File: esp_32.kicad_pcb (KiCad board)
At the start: 4 copper layers, 96 x 54 mm, 90 parts, among them J1 SS-52400-002, J3 GSD090012SEU, J4 B4B-XH-AM, J5 B2B-PH-SM4-TB, J6 Conn_01x05, Q1 TEMT6000X01, Q2 BC817, Q3 BC817, U1 MCP73871, U2 BME280, U3 ESP32-C3-WROOM-02-H4, U4 CP2102N-Axx-xQFN20, U5 USBLC6-2SC6, U6 W25Q32JVSSIQ, U7 MAX4466EXK

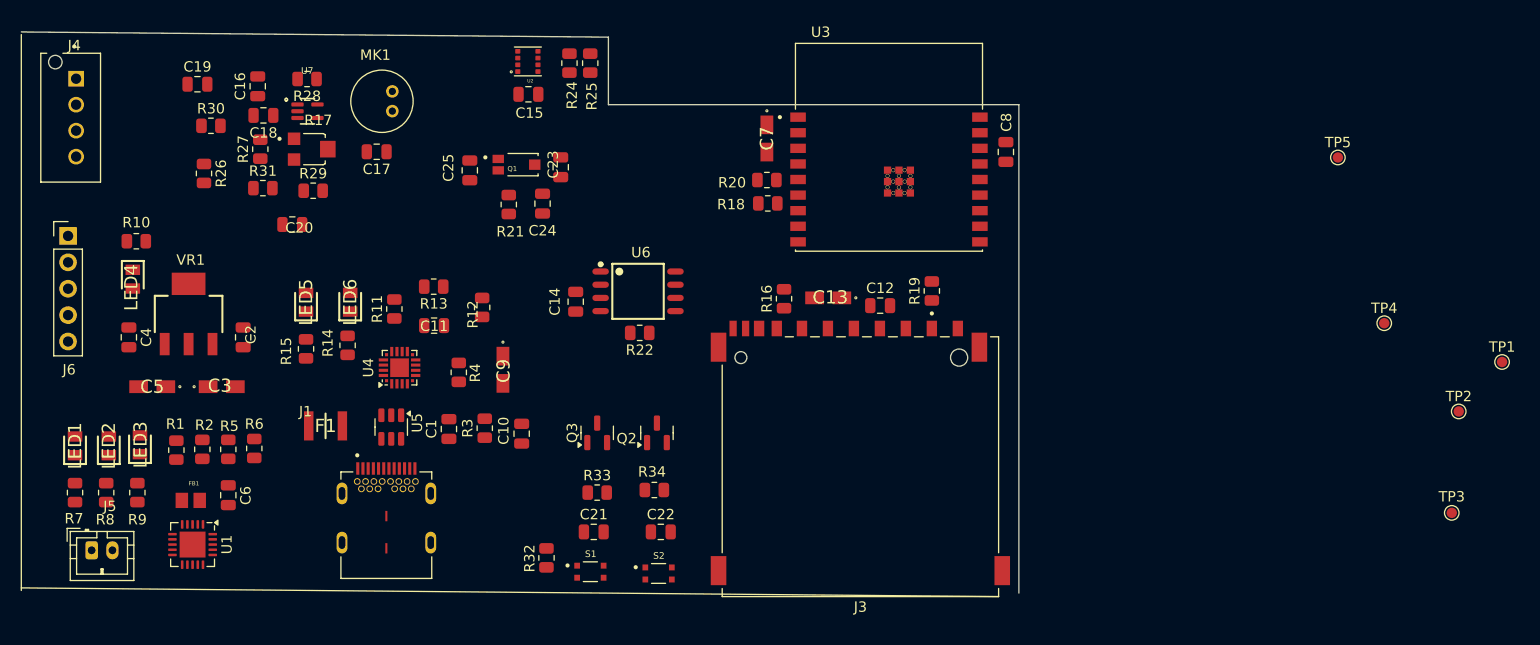
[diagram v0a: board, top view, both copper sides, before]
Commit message: PCB1
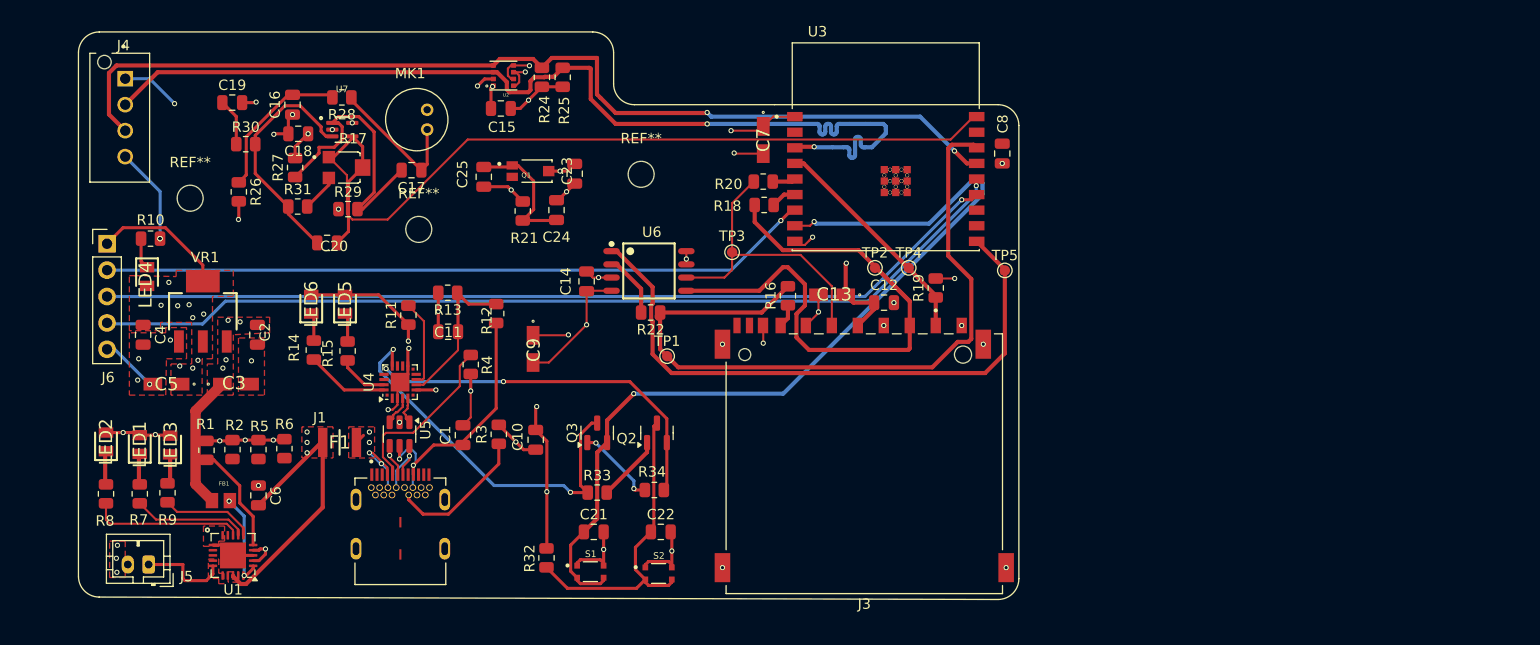
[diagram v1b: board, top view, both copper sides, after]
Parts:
- added REF**: MountingHole_2.5mm, MountingHole:MountingHole_2.5mm, F.Cu at (119.8, 98.5)
- added REF**: MountingHole_2.5mm, MountingHole:MountingHole_2.5mm, F.Cu at (163.2, 96.2)
- added REF**: MountingHole_2.5mm, MountingHole:MountingHole_2.5mm, F.Cu at (141.8, 101.5)
- moved TP1 80.4 mm to (165.7, 113.7)
- moved TP3 73.7 mm to (171.9, 103.7)
- moved TP2 57.9 mm to (185.7, 105.2)
- moved TP4 46.1 mm to (188.9, 105.2)
- moved TP5 33.8 mm to (198.2, 105.5)
- moved LED1 6.23 mm to (114.9, 122.2)
- moved R7 6.23 mm to (114.9, 127.0)
- moved J5 5.65 mm to (115.8, 133.8), turned to 180 degrees
- moved J4 4.72 mm to (113.0, 90.8)
- moved U1 4.03 mm to (123.9, 132.9), turned to 180 degrees
- moved R15 4.01 mm to (134.9, 113.2)
- moved J6 3.82 mm to (111.8, 102.9)
- moved C17 3.79 mm to (141.1, 95.8)
- moved C18 3.79 mm to (130.2, 92.3)
- moved R26 3.79 mm to (124.4, 97.9)
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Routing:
- net GND: track 0.00 -> 102.9 mm, vias 0 -> 44
- net /ESP32-c3-02/SDA: track 0.00 -> 97.9 mm, vias 0 -> 2
- net /ESP32-c3-02/SCL: track 0.00 -> 97.3 mm, vias 0 -> 2
- net /ESP32-c3-02/GPIO19: track 0.00 -> 90.3 mm, vias 0 -> 1
- net +3.3V: track 0.00 -> 90.3 mm, vias 0 -> 28
- net /ESP32-c3-02/GPIO18: track 0.00 -> 87.8 mm, vias 0 -> 1
- net /ESP32-c3-02/BOOT: track 0.00 -> 86.6 mm, vias 0 -> 2
- net /ESP32-c3-02/MIC_OUT: track 0.00 -> 86.0 mm
- net /ESP32-c3-02/MISO_DO: track 0.00 -> 72.1 mm
- net /ESP32-c3-02/GPIO8: track 0.00 -> 68.6 mm, vias 0 -> 1
- net /ESP32-c3-02/CS: track 0.00 -> 59.8 mm
- net /ESP32-c3-02/MOSI_DI: track 0.00 -> 58.2 mm
- net /ESP32-c3-02/DTR: track 0.00 -> 37.1 mm, vias 0 -> 2
- net /+5V_USB: track 0.00 -> 36.5 mm, vias 0 -> 6
- net /ESP32-c3-02/RTS: track 0.00 -> 36.0 mm, vias 0 -> 2
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- added copper zone on F.Cu, net +3.3V
- added copper zone on In1.Cu, net +3.3V
- added copper zone on F.Cu, net +5V
- added copper zone on F.Cu, net /+5V_USB
- added copper zone on In1.Cu, net /+5V_USB
- added copper zone on F.Cu, net /VBAT
- added copper zone on F.Cu, net /VBUS
- added copper zone on In1.Cu, net /VBUS
- added copper zone on F.Cu, net GND
- added copper zone on In2.Cu, net GND
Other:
- board outline removed

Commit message: finished_PCB
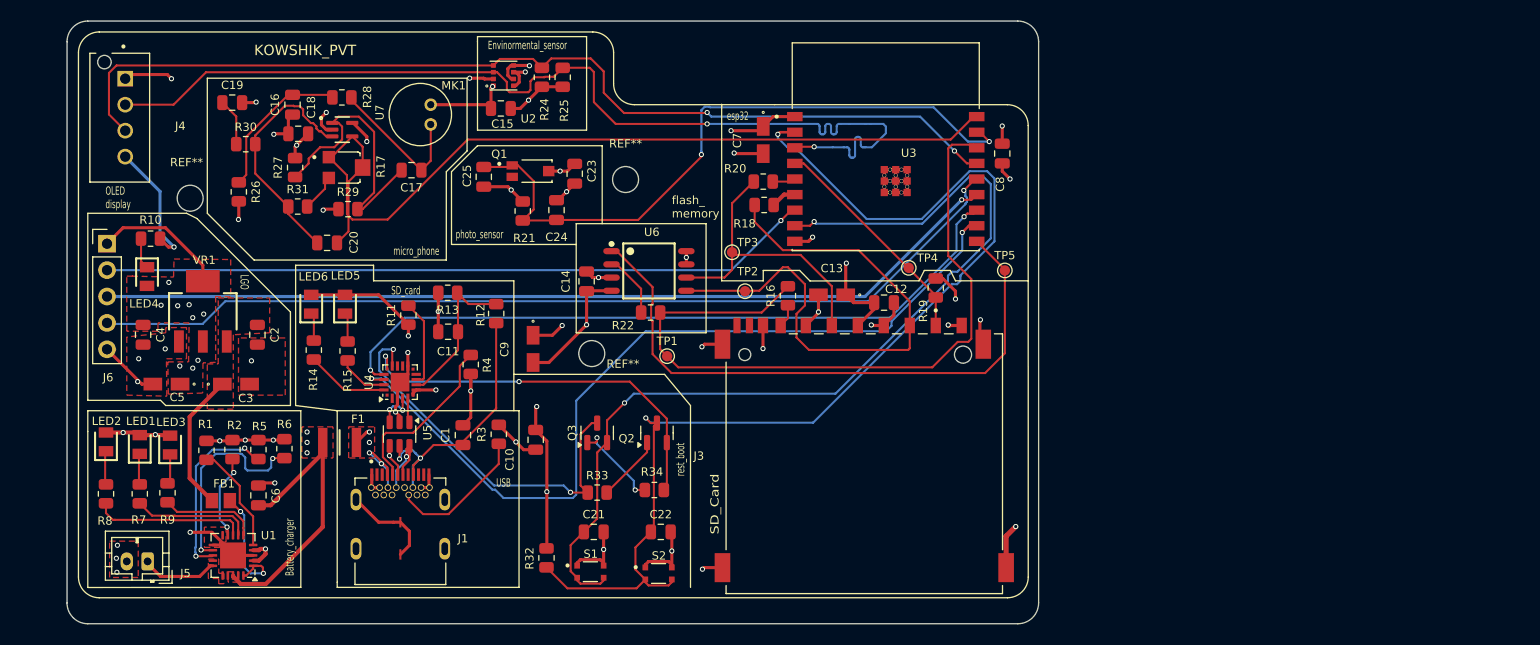
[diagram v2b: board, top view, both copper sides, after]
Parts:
- moved REF** 20.5 mm to (161.7, 96.7)
- moved REF** 17.9 mm to (158.4, 113.5)
- moved TP2 12.7 mm to (173.2, 107.5)
- moved MK1 0.60 mm to (141.9, 90.5)
- moved J5 0.32 mm to (115.7, 133.4)
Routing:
- net /ESP32-c3-02/TX_RX: track 0.00 -> 81.7 mm, vias 0 -> 2
- net /ESP32-c3-02/EN: track 30.3 -> 107.3 mm, vias 0 -> 2
- net /ESP32-c3-02/RX_TX: track 0.00 -> 68.7 mm, vias 0 -> 2
- net GND: track 102.9 -> 168.6 mm, vias 44 -> 40
- net /ESP32-c3-02/PHOTO_C: track 13.0 -> 64.7 mm, vias 0 -> 2
- net Net-(U1-PROG3): track 0.00 -> 19.8 mm, vias 0 -> 2
- net Net-(U1-PROG1): track 0.00 -> 18.0 mm, vias 0 -> 2
- net Net-(U1-~{TE}): track 0.00 -> 8.64 mm, vias 0 -> 2
- net /ESP32-c3-02/BOOT: track 86.6 -> 91.2 mm
- net +3.3V: track 90.3 -> 94.8 mm
- net Net-(FB1-Pad2): track 9.41 -> 13.0 mm
- net /ESP32-c3-02/MOSI_DI: track 58.2 -> 55.1 mm
- net /ESP32-c3-02/RTS: track 36.0 -> 38.5 mm
- net /+5V_USB: track 36.5 -> 38.2 mm
- net /VBAT: track 8.67 -> 7.09 mm
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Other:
- board outline added: 93.5 x 58 mm
- board text added: "Battery_charger"
- board text added: "Envinormental_sensor"
- board text added: "KOWSHIK_PVT"
- board text added: "LGO"
- board text added: "OLED display"
- board text added: "SD_Card"
- board text added: "SD_card"
- board text added: "USB"
- board text added: "esp32"
- board text added: "flash_ memory"
- board text added: "micro_phone"
- board text added: "photo_sensor"
- board text added: "rest_boot"
